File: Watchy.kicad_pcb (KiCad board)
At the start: 2 copper layers, 33.8 x 46 mm, 44 parts, among them J1 503480-0400, J2 Micro USB, J3 Battery, J4 FH33-10S-0.5SH_10_, M1 Vibration_Motor, Q2 UMH3N, Q4 CJ2301, Q5 S8050, SW1 BTN, SW2 BTN, SW3 BTN, SW4 BTN, U1 ESP32-PICO-D4, U10 BME280, U2 ME6211C33M5G-N, U3 CP2104, U4 BMA423, U5 TP4054, U7 MX25R3235FZNxx1, U8 L76-L, U9 IIS2MDCTR, Y1 RV-8523-C3-TA-QC-020

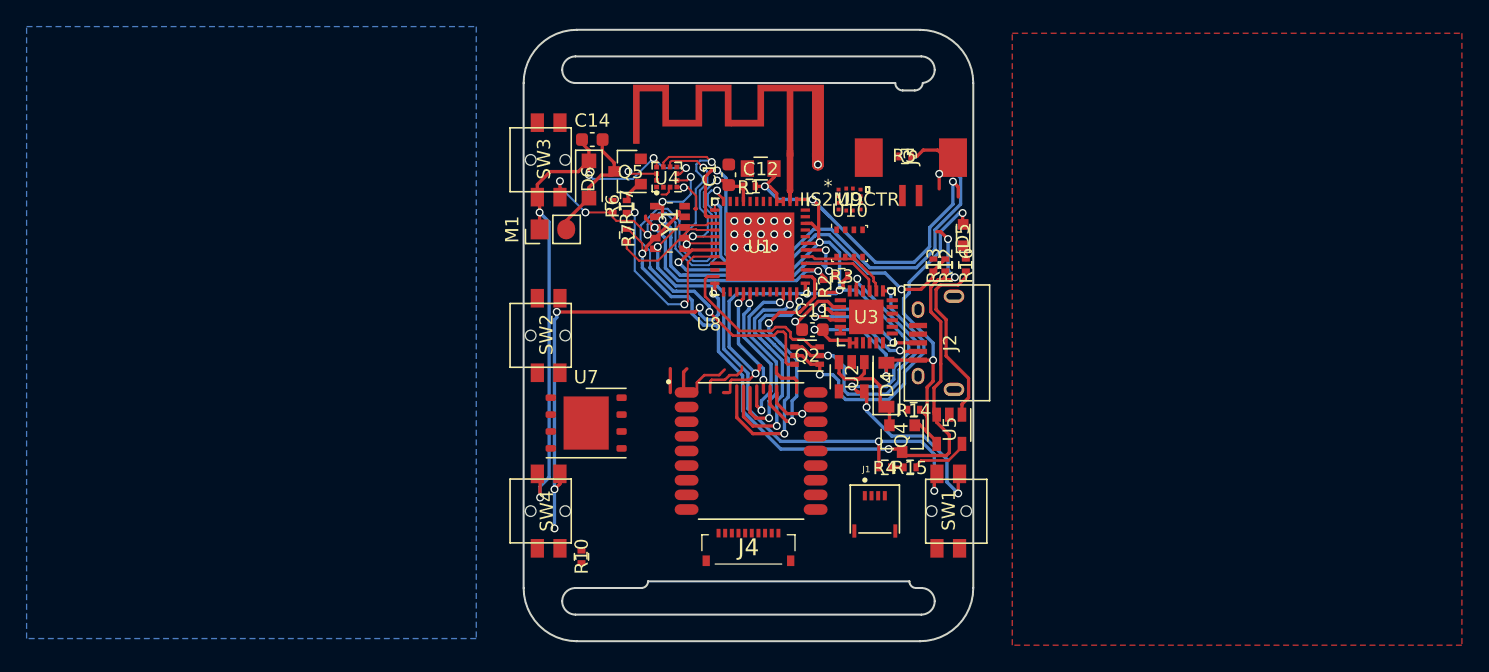
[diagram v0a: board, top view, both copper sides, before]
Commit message: version 0 production
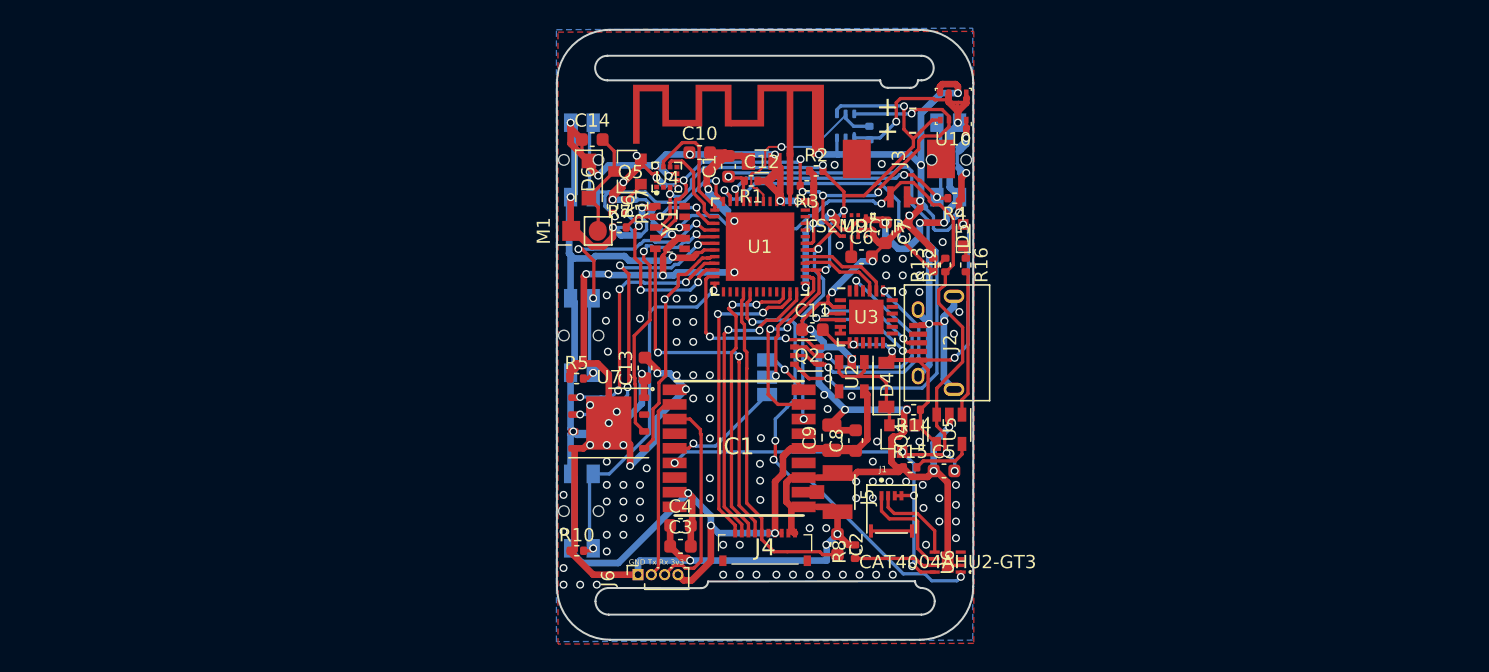
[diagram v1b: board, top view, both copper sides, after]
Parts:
- added C10: 100nF, Capacitor_SMD:C_0603_1608Metric, F.Cu at (81.9, 79.4)
- added C13: 100nF, Capacitor_SMD:C_0603_1608Metric, F.Cu at (77.8, 95.6)
- added C2: 100nF, Capacitor_SMD:C_0603_1608Metric, F.Cu at (92.3, 108.8)
- added C3: 1uF, Capacitor_SMD:C_0603_1608Metric, F.Cu at (80.5, 109.0)
- added C4: 100nF, Capacitor_SMD:C_0603_1608Metric, F.Cu at (80.5, 107.4)
- added C5: 100nF, Capacitor_SMD:C_0603_1608Metric, F.Cu at (100.3, 103.3)
- added C6: 220nF, Capacitor_SMD:C_0603_1608Metric, F.Cu at (94.1, 87.2)
- added C7: 220nF, Capacitor_SMD:C_0603_1608Metric, F.Cu at (95.9, 85.4)
- added C8: 100nF, Capacitor_SMD:C_0603_1608Metric, F.Cu at (93.7, 101.0)
- added C9: 10uF/50V, Capacitor_SMD:C_0805_2012Metric, F.Cu at (91.9, 100.8)
- added IC1: L76L-M33, Watchy:L76, F.Cu at (84.9, 101.6)
- added J5: U.FL-R-SMT(01), Watchy:HRS_U.FL-R-SMT(01), F.Cu at (92.3, 104.9)
- added J6: Conn_01x04_Female, Connector_PinSocket_1.00mm:PinSocket_1x04_P1.00mm_Vertical, F.Cu at (77.3, 111.1)
- added JP1: SolderJumper_3_Open, Jumper:SolderJumper-3_P1.3mm_Open_Pad1.0x1.5mm, B.Cu at (87.0, 96.3)
- added R8: 3.5K, Resistor_SMD:R_0402_1005Metric, F.Cu at (93.6, 109.4)
- added R9: 10K, Resistor_SMD:R_0402_1005Metric, B.Cu at (94.7, 77.9)
- added U6: CAT4004AHU2-GT3, Watchy:CAT4004AHU2-GT3, F.Cu at (100.6, 110.2)
- J4: value FH33-10S-0.5SH_10_ -> FH33-10S-0.5SH(10)
- R1, R10, R12, R13, R14, R15, R16, R17, R2, R3, R4, R5, R6, R7: footprint Resistors_SMD:R_0402 -> Resistor_SMD:R_0402_1005Metric
- SW1, SW2, SW3, SW4: moved to B.Cu
- U7: value MX25R3235FZNxx1 -> MX25L25645GZN-10G
- U8: value L76-L -> LTR-303ALS-01; footprint Watchy:XCVR_L76-L -> OptoDevice:Lite-On_LTR-303ALS-01; moved to B.Cu
- moved R5 29.8 mm to (72.7, 96.4)
- moved SW1 26.4 mm to (100.7, 79.9), turned to 90 degrees
- moved U8 25.4 mm to (92.9, 77.4), turned to 90 degrees
- moved R4 20.9 mm to (101.1, 82.8)
- moved U10 12.9 mm to (101.0, 75.9), turned to 180 degrees
- moved R2 8.70 mm to (90.7, 80.8), turned to 0 degrees
- moved R3 7.24 mm to (90.0, 81.9)
- moved SW2 2.50 mm to (73.0, 93.1), turned to 270 degrees
- moved SW3 2.50 mm to (73.0, 79.9), turned to 270 degrees
- moved SW4 2.50 mm to (73.0, 106.3), turned to 270 degrees
- moved M1 2.38 mm to (72.3, 85.3)
- moved U9 2.04 mm to (93.6, 84.9)
- moved U7 1.70 mm to (75.1, 99.7)
- moved J1 1.25 mm to (96.3, 106.5)
- moved J4 1.25 mm to (86.8, 110.3)
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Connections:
- J1 pad 1: (no net) -> Net-(J1-Pad1)
- J1 pad 2: (no net) -> Net-(J1-Pad2)
- J1 pad 3: (no net) -> +BATT
- J1 pad 4: (no net) -> +BATT
- J4 pad 1: (no net) -> LCD_CLK
- J4 pad 10: (no net) -> GND
- J4 pad 2: (no net) -> LCD_MOSI
- J4 pad 3: (no net) -> LCD_CS
- J4 pad 4: (no net) -> EXTCOM
- J4 pad 5: (no net) -> LCD_EN
- J4 pad 6: (no net) -> +3V3
- J4 pad 7: (no net) -> +3V3
- J4 pad 8: (no net) -> +3V3
- J4 pad 9: (no net) -> GND
- R7 pad 1: +BATT -> +3V3
- R7 pad 2: RTC_INT -> INT_RTC
- U1 pad 10: (no net) -> BTN_1
- U1 pad 11: (no net) -> ADC
- U1 pad 13: ADC -> INT_ACC2
- U1 pad 14: BTN_2 -> INT_ACC1
- U1 pad 15: BTN_1 -> INT_RTC
- U1 pad 16: RTC_INT -> BTN_2
- U1 pad 17: ACC_INT_1 -> FLASH_CLK
- U1 pad 18: ACC_INT_2 -> FLASH_MISO
- U1 pad 20: VIB_PWM -> FLASH_MOSI
- U1 pad 21: GND -> FLASH_CS
- U1 pad 22: (no net) -> VIB_PWM
- U1 pad 28: (no net) -> LCD_EN
- U1 pad 29: (no net) -> BL_PWM
- U1 pad 34: (no net) -> LCD_CS
- U1 pad 35: (no net) -> LCD_CLK
- U1 pad 36: (no net) -> LCD_MOSI
- U1 pad 38: (no net) -> GPS_FORCE_ON
- U1 pad 6: (no net) -> INT_ALS
- U10 pad 1: (no net) -> GND
- U10 pad 2: (no net) -> +3V3
- U10 pad 3: (no net) -> SDA
- U10 pad 4: (no net) -> SCL
- U10 pad 5: (no net) -> GND
- U10 pad 6: (no net) -> +3V3
- U10 pad 7: (no net) -> GND
- U10 pad 8: (no net) -> +3V3
- U4 pad 5: ACC_INT_1 -> INT_ACC1
- U4 pad 6: ACC_INT_2 -> INT_ACC2
- U7 pad 1: (no net) -> FLASH_CS
- U7 pad 2: (no net) -> FLASH_MISO
- U7 pad 3: (no net) -> +3V3
- U7 pad 4: Net-(U7-Pad4) -> GND
- U7 pad 5: (no net) -> FLASH_MOSI
- U7 pad 6: (no net) -> FLASH_CLK
- U7 pad 8: (no net) -> +3V3
- U7 pad 9: Net-(U7-Pad4) -> GND
- U8 pad 1: Net-(U8-Pad1) -> +3V3
- U8 pad 3: (no net) -> GND
- U8 pad 4: (no net) -> SCL
- U8 pad 5: (no net) -> INT_ALS
- U8 pad 6: (no net) -> SDA
- U9 pad 1: (no net) -> SCL
- U9 pad 10: (no net) -> +3V3
- U9 pad 3: (no net) -> +3V3
- U9 pad 4: (no net) -> SDA
- U9 pad 5: (no net) -> Net-(C6-Pad1)
- U9 pad 6: (no net) -> GND
- U9 pad 8: (no net) -> GND
- U9 pad 9: (no net) -> +3V3
- Y1 pad 1: (no net) -> +3V3
- Y1 pad 2: (no net) -> INT_RTC
- Y1 pad 3: (no net) -> SCL
- Y1 pad 4: (no net) -> SDA
- Y1 pad 5: (no net) -> EXTCOM
- Y1 pad 7: (no net) -> GND
- Y1 pad 8: (no net) -> +BATT
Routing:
- net GND: track 18.4 -> 314.3 mm, vias 19 -> 134
- net +3V3: track 149.6 -> 253.3 mm, vias 16 -> 25
- net (no net): track 94.6 -> 0.00 mm, vias 12 -> 0
- net SCL: track 19.6 -> 61.9 mm, vias 2 -> 7
- net BL_PWM: track 0.00 -> 35.2 mm, vias 0 -> 4
- net SDA: track 27.9 -> 61.7 mm, vias 5 -> 8
- net EXTCOM: track 0.00 -> 27.9 mm, vias 0 -> 2
- net LCD_EN: track 0.00 -> 25.5 mm
- net LCD_CS: track 0.00 -> 24.2 mm, vias 0 -> 2
- net LCD_CLK: track 0.00 -> 23.4 mm, vias 0 -> 2
- net LCD_MOSI: track 0.00 -> 22.8 mm, vias 0 -> 2
- net FLASH_MISO: track 0.00 -> 22.7 mm, vias 0 -> 4
- net BTN_2: track 43.2 -> 22.4 mm, vias 2 -> 4
- net FLASH_CLK: track 0.00 -> 20.7 mm, vias 0 -> 2
- net BTN_1: track 43.3 -> 24.0 mm
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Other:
- board size 33.8 x 46 mm -> 31.3 x 45.8 mm
- board text added: "+ -"
- board text added: "ATGM module"
- board text added: "GND Tx Rx 3v3"
- board text added: "Quectel module"
- board text added: "watchy-sports Modified from Watchy (US000936) (2021)"
- board text removed: "watchy"

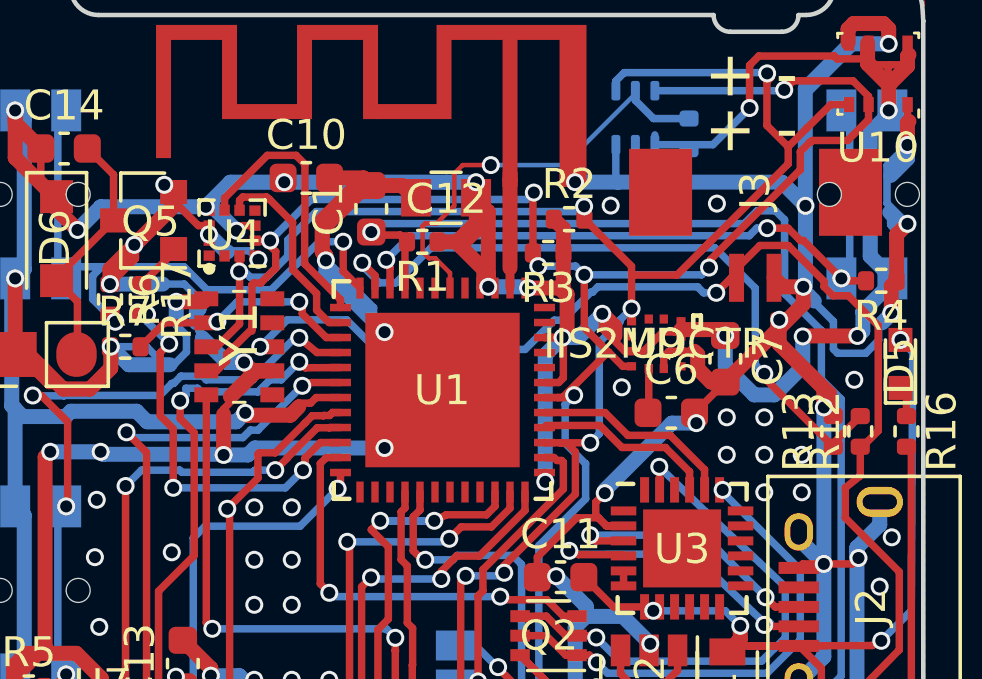
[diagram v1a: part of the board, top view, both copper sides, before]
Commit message: v0 PCBWay final version
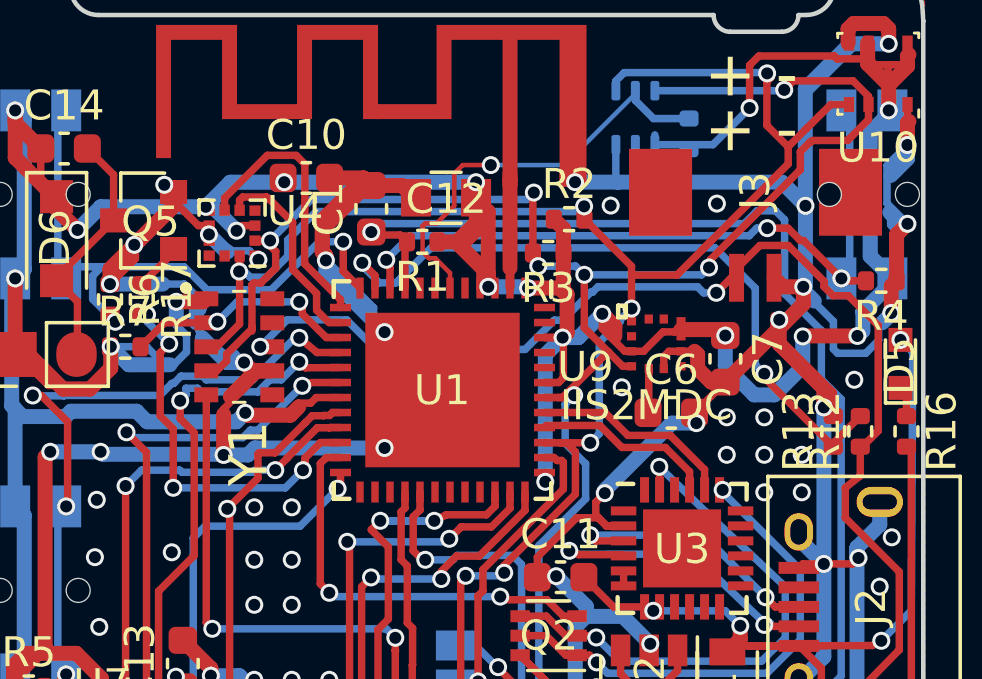
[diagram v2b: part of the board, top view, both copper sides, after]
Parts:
- U9: value IIS2MDCTR -> IIS2MDC
